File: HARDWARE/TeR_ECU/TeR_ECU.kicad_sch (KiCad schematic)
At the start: 6 parts

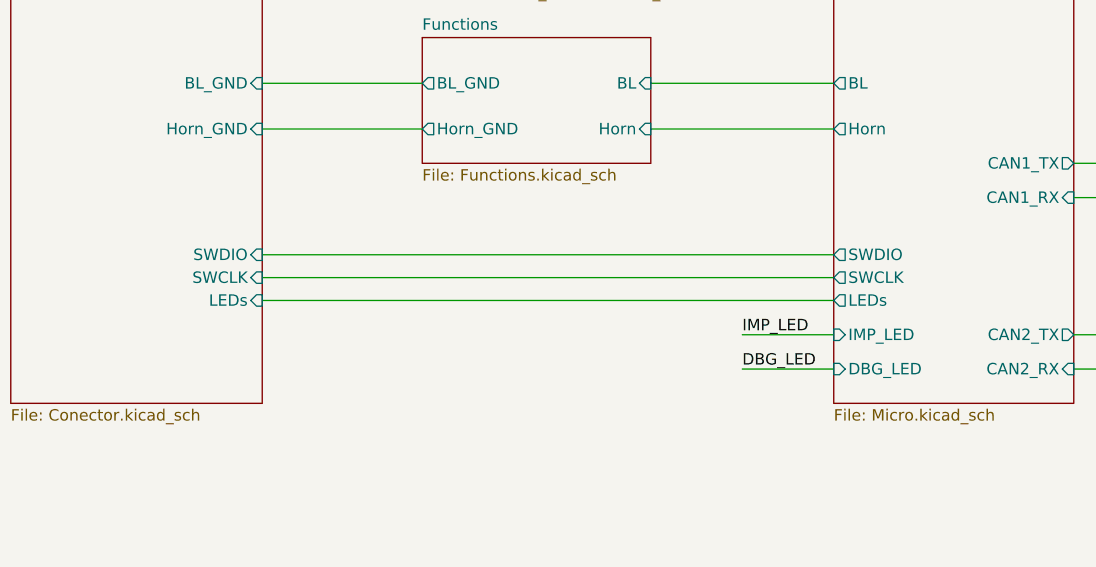
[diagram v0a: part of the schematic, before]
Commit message: Solo falta revisar
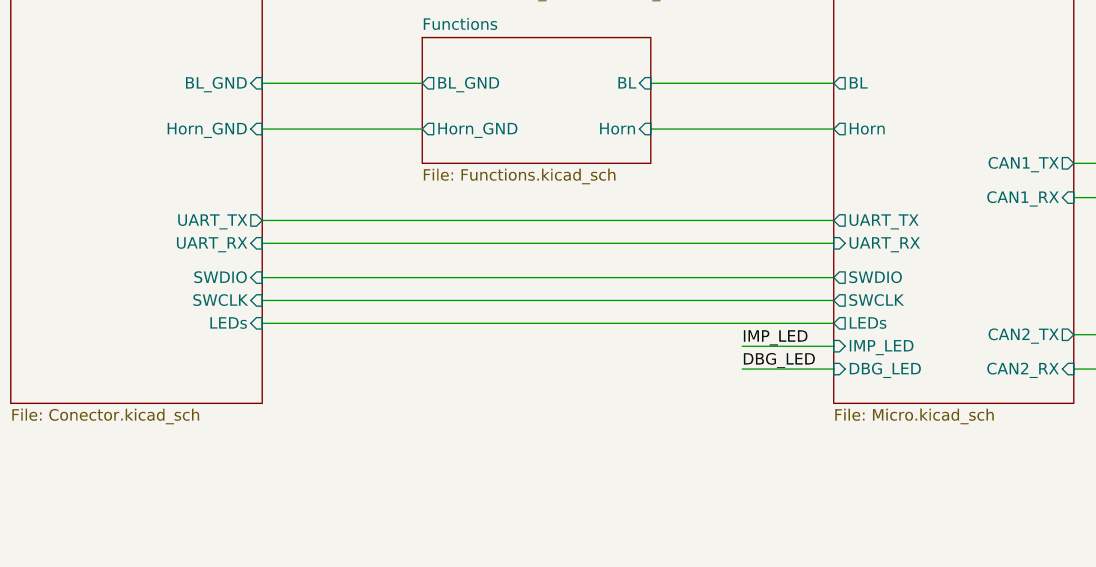
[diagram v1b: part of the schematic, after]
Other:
- sheet Conector ports: added UART_RX, UART_TX; removed none
- sheet Micro ports: added UART_RX, UART_TX; removed none
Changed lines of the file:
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@@
+    (stroke (width 0) (type default))
+  )
+  (wire (pts (xy 66.04 118.11) (xy 129.54 118.11))
     (stroke (width 0) (type default))
   )
@@
     (stroke (width 0) (type default))
   )
+  (wire (pts (xy 66.04 115.57) (xy 129.54 115.57))
+    (stroke (width 0) (type default))
+  )
   (wire (pts (xy 109.22 81.28) (xy 129.54 81.28))
     (stroke (width 0) (type default))
@@
     (stroke (width 0) (type default))
   )
+  (wire (pts (xy 66.04 127) (xy 129.54 127))
+    (stroke (width 0) (type default))
+  )
+  (wire (pts (xy 109.22 100.33) (xy 129.54 100.33))
+    (stroke (width 0) (type default))
+  )
+  (wire (pts (xy 218.44 109.22) (xy 223.52 109.22))
+    (stroke (width 0) (type default))
+  )
+  (wire (pts (xy 119.38 129.54) (xy 129.54 129.54))
+    (stroke (width 0) (type default))
+  )
+  (wire (pts (xy 66.04 81.28) (xy 83.82 81.28))
+    (stroke (width 0) (type default))
+  )
   (wire (pts (xy 66.04 124.46) (xy 129.54 124.46))
     (stroke (width 0) (type default))
   )
-  (wire (pts (xy 109.22 100.33) (xy 129.54 100.33))
-    (stroke (width 0) (type default))
-  )
-  (wire (pts (xy 218.44 109.22) (xy 223.52 109.22))
-    (stroke (width 0) (type default))
-  )
-  (wire (pts (xy 119.38 128.27) (xy 129.54 128.27))
-    (stroke (width 0) (type default))
-  )
-  (wire (pts (xy 66.04 81.28) (xy 83.82 81.28))
-    (stroke (width 0) (type default))
-  )
   (wire (pts (xy 66.04 121.92) (xy 129.54 121.92))
-    (stroke (width 0) (type default))
-  )
-  (wire (pts (xy 66.04 119.38) (xy 129.54 119.38))
     (stroke (width 0) (type default))
   )
@@
     (effects (font (size 1.27 1.27)) (justify left bottom))
   )
-  (label "IMP_LED" (at 119.38 128.27 0) (fields_autoplaced)
+  (label "IMP_LED" (at 119.38 129.54 0) (fields_autoplaced)
     (effects (font (size 1.27 1.27)) (justify left bottom))
   )
@@
       (effects (font (size 1.27 1.27)) (justify left))
     )
-    (pin "IMP_LED" input (at 129.54 128.27 180)
+    (pin "IMP_LED" input (at 129.54 129.54 180)
       (effects (font (size 1.27 1.27)) (justify left))
     )
@@
       (effects (font (size 1.27 1.27)) (justify left))
     )
-    (pin "LEDs" output (at 129.54 124.46 180)
-      (effects (font (size 1.27 1.27)) (justify left))
-    )
-    (pin "SWCLK" output (at 129.54 121.92 180)
-      (effects (font (size 1.27 1.27)) (justify left))
-    )
-    (pin "SWDIO" output (at 129.54 119.38 180)
+    (pin "LEDs" output (at 129.54 127 180)
+      (effects (font (size 1.27 1.27)) (justify left))
+    )
+    (pin "SWCLK" output (at 129.54 124.46 180)
+      (effects (font (size 1.27 1.27)) (justify left))
+    )
+    (pin "SWDIO" output (at 129.54 121.92 180)
+      (effects (font (size 1.27 1.27)) (justify left))
+    )
+    (pin "UART_RX" input (at 129.54 118.11 180)
+      (effects (font (size 1.27 1.27)) (justify left))
+    )
+    (pin "UART_TX" output (at 129.54 115.57 180)
       (effects (font (size 1.27 1.27)) (justify left))
     )
@@
       (effects (font (size 1.27 1.27)) (justify right))
     )
-    (pin "LEDs" input (at 66.04 124.46 0)
-      (effects (font (size 1.27 1.27)) (justify right))
-    )
-    (pin "SWCLK" input (at 66.04 121.92 0)
-      (effects (font (size 1.27 1.27)) (justify right))
-    )
-    (pin "SWDIO" input (at 66.04 119.38 0)
-      (effects (font (size 1.27 1.27)) (justify right))
-    )
+    (pin "LEDs" input (at 66.04 127 0)
+      (effects (font (size 1.27 1.27)) (justify right))
+    )
+    (pin "SWCLK" input (at 66.04 124.46 0)
+      (effects (font (size 1.27 1.27)) (justify right))
+    )
+    (pin "SWDIO" input (at 66.04 121.92 0)
+      (effects (font (size 1.27 1.27)) (justify right))
+    )
+    (pin "UART_RX" input (at 66.04 118.11 0)
+      (effects (font (size 1.27 1.27)) (justify right))
+    )
+    (pin "UART_TX" output (at 66.04 115.57 0)
+      (effects (font (size 1.27 1.27)) (justify right))
+    )
